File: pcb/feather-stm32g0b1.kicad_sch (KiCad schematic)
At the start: 22 parts, among them SW1 SW_Push, U1 STM32G0B1CBT6, Y1 32.768 KHz, 10ppm, 12.5pf, Y2 8 MHz, 10ppm, 10pf

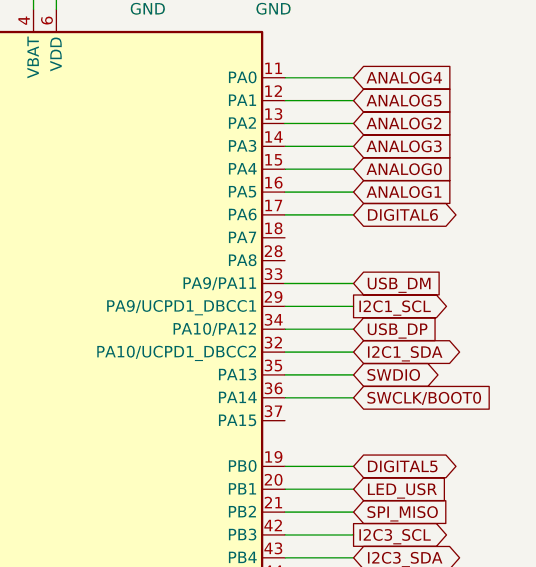
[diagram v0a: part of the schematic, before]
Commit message: More PCB layout updates
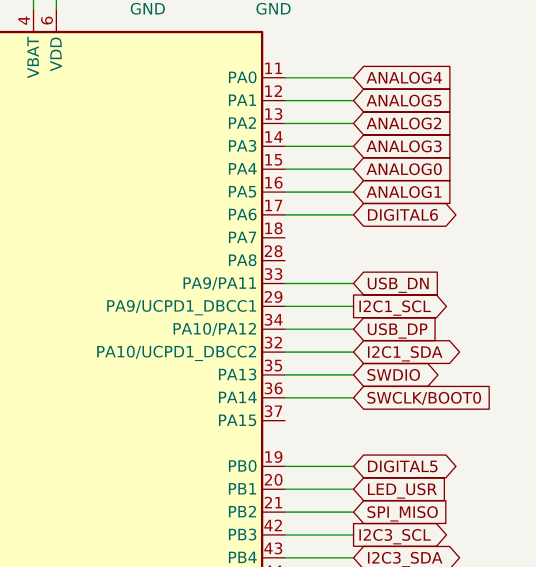
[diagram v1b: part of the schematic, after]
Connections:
- net USB_DM renamed USB_DN
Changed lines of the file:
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@@
 		)
 	)
-	(global_label "USB_DM"
+	(global_label "USB_DN"
 		(shape input)
 		(at 260.35 69.85 0)
@@
 		)
 		(property "Intersheetrefs" "${INTERSHEET_REFS}"
-			(at 270.8342 69.85 0)
+			(at 270.7133 69.85 0)
 			(effects
 				(font
